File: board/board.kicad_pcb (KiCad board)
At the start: 2 copper layers, 21 x 13 mm, 1 part

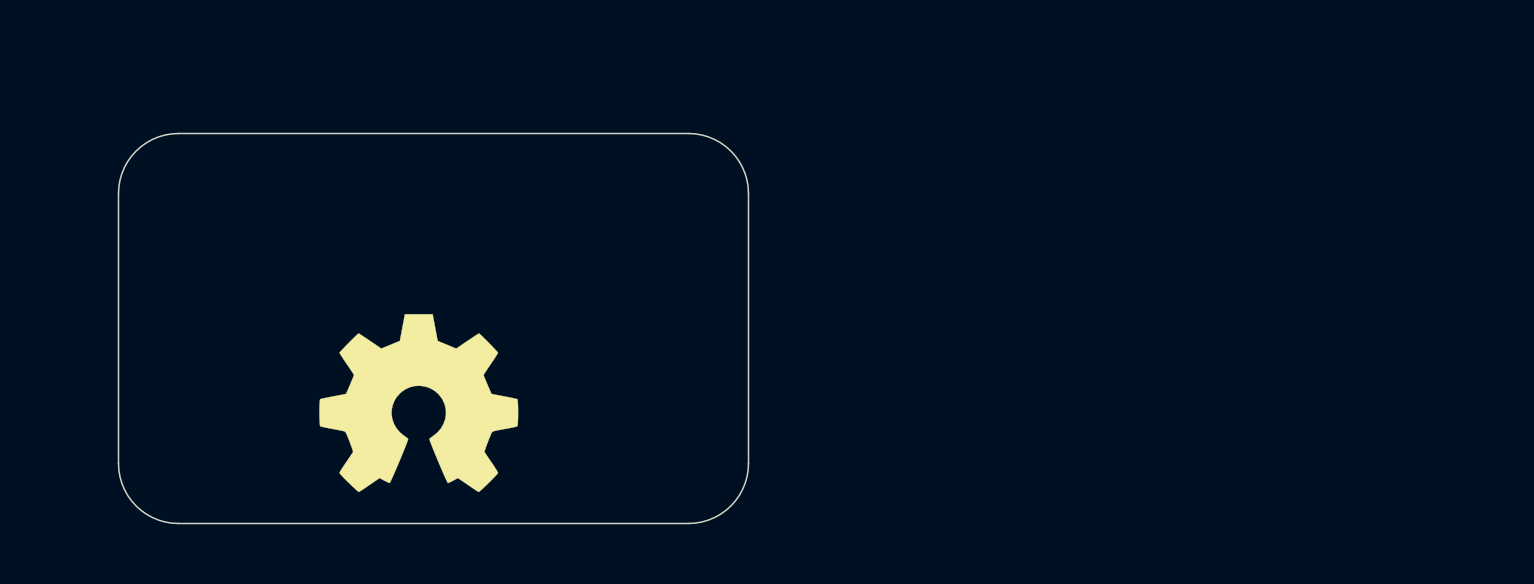
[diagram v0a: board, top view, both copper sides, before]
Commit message: initial
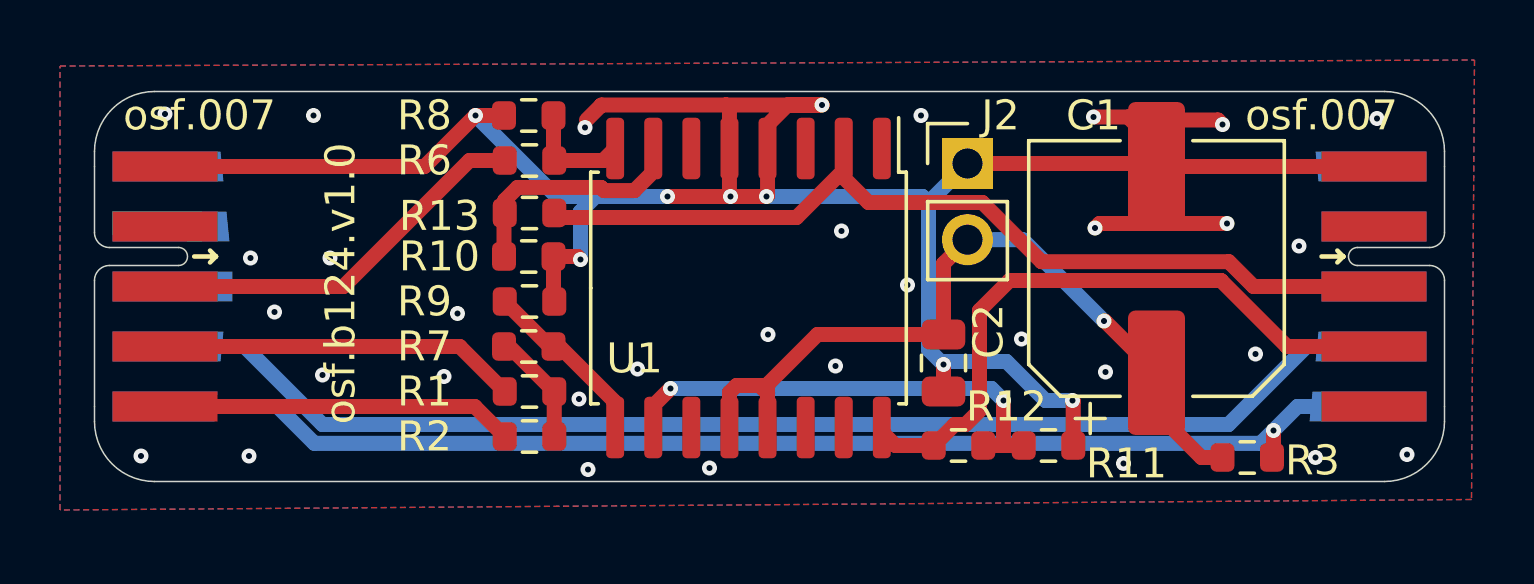
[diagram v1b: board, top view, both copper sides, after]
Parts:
- added C1: 100uF, Capacitor_SMD:CP_Elec_8x6.9, F.Cu at (174.6, 94.5)
- added C2: 1uF, Capacitor_SMD:C_0805_2012Metric, F.Cu at (167.5, 97.7)
- added J1: 007_ADC, on_edge:on_edge_2x05_device, F.Cu at (139.2, 95.1)
- added J2: Conn_01x02_Male, Connector_PinHeader_2.54mm:PinHeader_1x02_P2.54mm_Vertical, F.Cu at (168.3, 91.0)
- added J3: 007_ADC, on_edge:on_edge_2x05_host, F.Cu at (184.2, 95.1)
- added R1: 0R, Resistor_SMD:R_0603_1608Metric, F.Cu at (153.7, 98.6)
- added R10: d.n.p, Resistor_SMD:R_0603_1608Metric, F.Cu at (153.7, 94.1)
- added R11: d.n.p, Resistor_SMD:R_0603_1608Metric, F.Cu at (171.0, 100.4)
- added R12: 0R, Resistor_SMD:R_0603_1608Metric, F.Cu at (168.0, 100.4)
- added R13: 0R, Resistor_SMD:R_0603_1608Metric, F.Cu at (153.7, 92.7)
- added R2: 0R, Resistor_SMD:R_0603_1608Metric, F.Cu at (153.7, 100.1)
- added R3: 0R, Resistor_SMD:R_0603_1608Metric, F.Cu at (177.6, 100.8)
- added R6: 0R, Resistor_SMD:R_0603_1608Metric, F.Cu at (153.7, 90.9)
- added R7: 0R, Resistor_SMD:R_0603_1608Metric, F.Cu at (153.7, 97.1)
- added R8: d.n.p, Resistor_SMD:R_0603_1608Metric, F.Cu at (153.7, 89.4)
- added R9: d.n.p, Resistor_SMD:R_0603_1608Metric, F.Cu at (153.7, 95.6)
- added U1: TCA0372, Package_SO:SOIC-16W_7.5x10.3mm_P1.27mm, F.Cu at (161.0, 95.2)
- LOGO1: moved to B.Cu
- moved LOGO1 11.7 mm to (161.0, 95.2), turned to 180 degrees
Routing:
- net GND: track 0.00 -> 93.0 mm, vias 0 -> 40
- net Net-(J1-Pad9): track 0.00 -> 42.4 mm
- net Net-(J1-Pad10): track 0.00 -> 42.1 mm, vias 0 -> 1
- net /implementation/out1: track 0.00 -> 31.3 mm
- net /VDD: track 0.00 -> 26.4 mm, vias 0 -> 1
- net /implementation/out2: track 0.00 -> 21.9 mm
- net Net-(R11-Pad2): track 0.00 -> 15.7 mm, vias 0 -> 2
- net /implementation/in1: track 0.00 -> 13.1 mm
- net Net-(J1-Pad4): track 0.00 -> 11.9 mm
- net Net-(J1-Pad5): track 0.00 -> 11.7 mm
- net Net-(R10-Pad2): track 0.00 -> 8.09 mm
- net Net-(R7-Pad1): track 0.00 -> 5.91 mm
- net /implementation/in2: track 0.00 -> 3.80 mm
- net Net-(R6-Pad1): track 0.00 -> 3.71 mm
- added copper zone on B.Cu, net GND
- added copper zone on F.Cu, net GND
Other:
- board size 21 x 13 mm -> 45 x 13 mm
- board text added: "osf.007"
- board text added: "osf.b124.v1.0"
